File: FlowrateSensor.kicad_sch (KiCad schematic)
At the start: 21 parts, among them Q3 PSMN8R5-40MSDX, U6 TPS5405DR

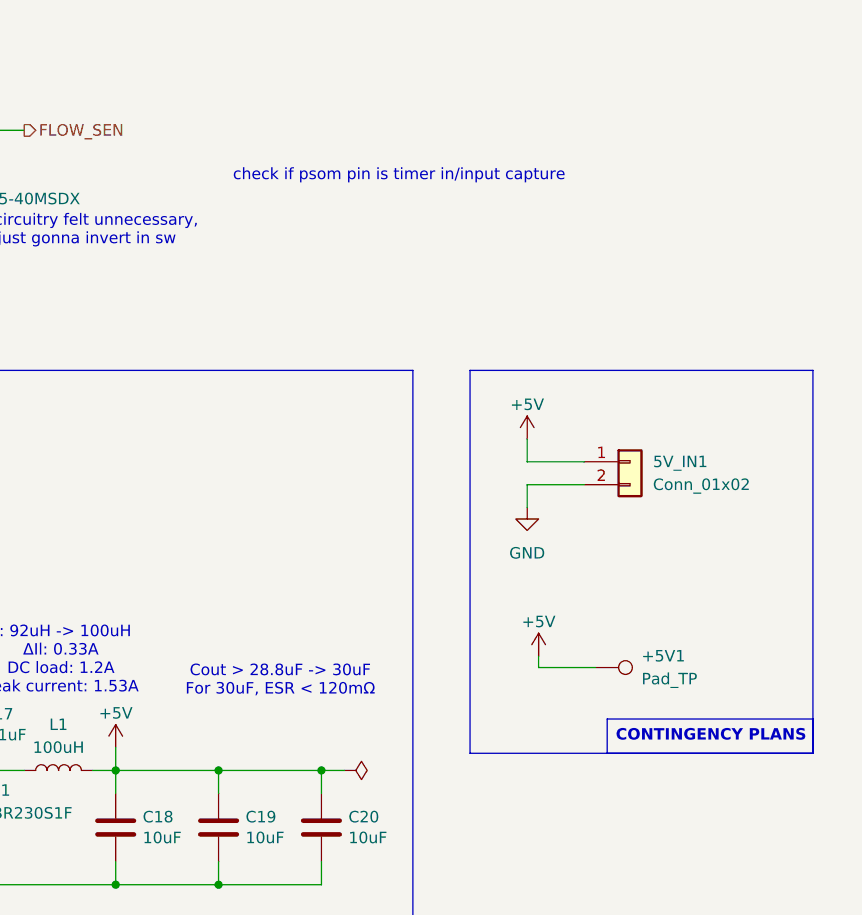
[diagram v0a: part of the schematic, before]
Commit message: datasheets disappeared for some reason
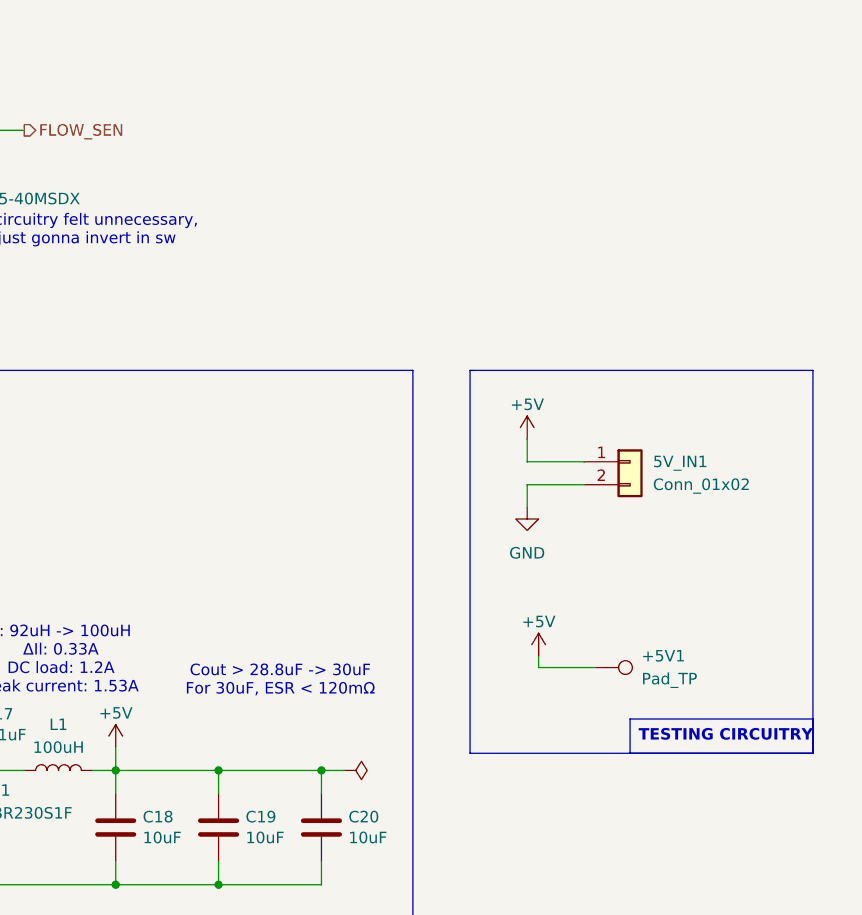
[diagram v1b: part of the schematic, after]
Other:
- note removed: "check if psom pin is timer in/input capture"
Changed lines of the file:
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@@
-		)
-	)
-	(text "check if psom pin is timer in/input capture"
-		(exclude_from_sim no)
-		(at 182.626 41.91 0)
-		(effects
-			(font
-				(size 1.27 1.27)
-			)
 		)
 	)
@@
 		)
 	)
-	(text_box "CONTINGENCY PLANS"
+	(text_box "TESTING CIRCUITRY"
 		(exclude_from_sim no)
-		(at 205.74 102.235 0)
-		(size 22.86 3.81)
+		(at 208.28 102.235 0)
+		(size 20.32 3.81)
 		(margins 0.9525 0.9525 0.9525 0.9525)
 		(stroke
